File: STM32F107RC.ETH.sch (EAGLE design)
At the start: 30 parts, among them J1 HR911105A, Q1 8MHz, U1 LAN8720A-CP, U2 STM32F107RCT6, X1 CB3LV-3I-74M2500

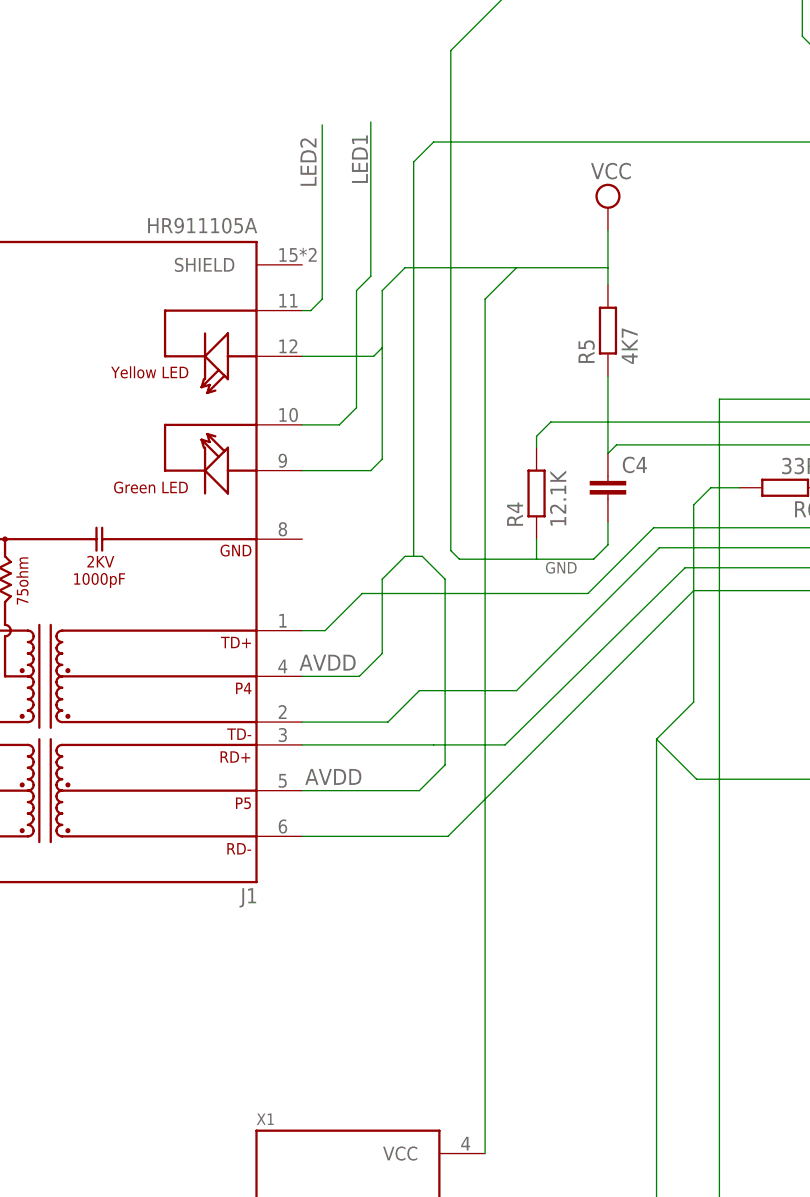
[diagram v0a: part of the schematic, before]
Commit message: Add files via upload
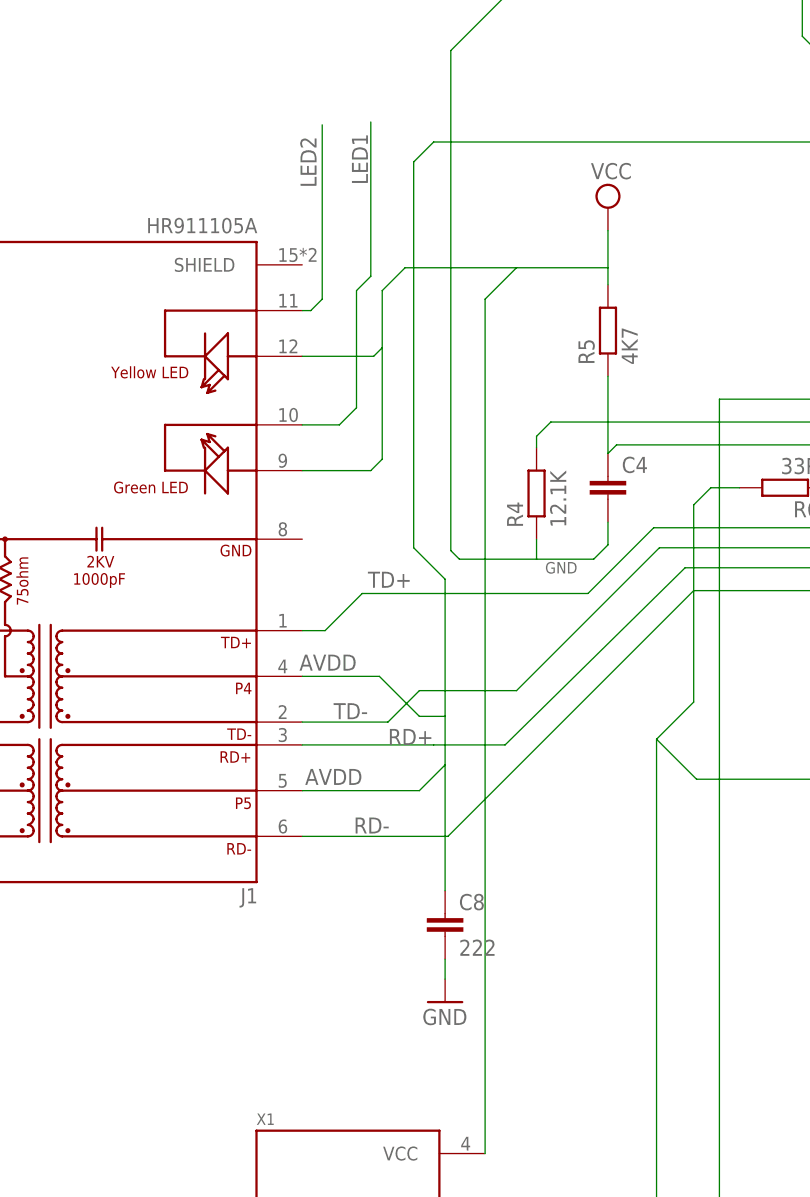
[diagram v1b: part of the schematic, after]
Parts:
- added C8: 222, resistor:C-EUC1206
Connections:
- net N$23 renamed TD+
- net N$28 renamed TD-
- net N$29 renamed RD+
- net N$31 renamed RD-
- net AVDD: now also C8.1
- net GND: now also C8.2
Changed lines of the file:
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@@
 <part name="R13" library="resistor" deviceset="R-EU_" device="0204_7" value="330R"/>
 <part name="R14" library="resistor" deviceset="R-EU_" device="0204_7" value="330R"/>
+<part name="C8" library="resistor" deviceset="C-EU" device="C1206" value="222"/>
+<part name="GND1" library="supply1" deviceset="GND" device=""/>
 </parts>
 <sheets>
@@
 <instance part="R13" gate="G$1" x="-12.3825" y="124.46"/>
 <instance part="R14" gate="G$1" x="-12.3825" y="117.475"/>
+<instance part="C8" gate="G$1" x="-104.14" y="100.33"/>
+<instance part="GND1" gate="1" x="-104.14" y="90.4875"/>
 </instances>
 <busses>
@@
 <junction x="0" y="195.58"/>
 <label x="-9.8425" y="196.5325" size="1.778" layer="95"/>
-<wire x1="-113.665" y1="126.6825" x2="-111.125" y2="129.2225" width="0.1524" layer="91"/>
 <pinref part="J1" gate="G$1" pin="P4"/>
-<wire x1="-120.015" y1="126.6825" x2="-113.665" y2="126.6825" width="0.1524" layer="91"/>
-<wire x1="-111.125" y1="129.2225" x2="-111.125" y2="137.4775" width="0.1524" layer="91"/>
-<wire x1="-111.125" y1="137.4775" x2="-108.585" y2="140.0175" width="0.1524" layer="91"/>
-<wire x1="-104.14" y1="137.4775" x2="-106.68" y2="140.0175" width="0.1524" layer="91"/>
-<wire x1="-104.14" y1="116.84" x2="-104.14" y2="137.4775" width="0.1524" layer="91"/>
+<wire x1="-120.015" y1="126.6825" x2="-111.4425" y2="126.6825" width="0.1524" layer="91"/>
+<wire x1="-104.14" y1="137.4775" x2="-107.6325" y2="140.97" width="0.1524" layer="91"/>
+<wire x1="-104.14" y1="116.84" x2="-104.14" y2="122.2375" width="0.1524" layer="91"/>
 <pinref part="J1" gate="G$1" pin="P5"/>
+<wire x1="-104.14" y1="122.2375" x2="-104.14" y2="137.4775" width="0.1524" layer="91"/>
 <wire x1="-120.015" y1="113.9825" x2="-106.9975" y2="113.9825" width="0.1524" layer="91"/>
 <wire x1="-106.9975" y1="113.9825" x2="-104.14" y2="116.84" width="0.1524" layer="91"/>
-<wire x1="-108.585" y1="140.0175" x2="-107.6325" y2="140.0175" width="0.1524" layer="91"/>
-<wire x1="-107.6325" y1="140.0175" x2="-106.68" y2="140.0175" width="0.1524" layer="91"/>
-<wire x1="-107.6325" y1="140.0175" x2="-107.6325" y2="183.8325" width="0.1524" layer="91"/>
+<wire x1="-107.6325" y1="140.97" x2="-107.6325" y2="183.8325" width="0.1524" layer="91"/>
 <wire x1="-107.6325" y1="183.8325" x2="-105.41" y2="186.055" width="0.1524" layer="91"/>
 <wire x1="-105.41" y1="186.055" x2="-33.02" y2="186.055" width="0.1524" layer="91"/>
@@
 <label x="-120.3325" y="127.3175" size="1.778" layer="95"/>
 <label x="-119.6975" y="114.6175" size="1.778" layer="95"/>
+<wire x1="-111.4425" y1="126.6825" x2="-106.9975" y2="122.2375" width="0.1524" layer="91"/>
+<wire x1="-106.9975" y1="122.2375" x2="-104.14" y2="122.2375" width="0.1524" layer="91"/>
+<wire x1="-104.14" y1="116.84" x2="-104.14" y2="102.87" width="0.1524" layer="91"/>
+<pinref part="C8" gate="G$1" pin="1"/>
 </segment>
 </net>
@@
 <wire x1="29.845" y1="151.4475" x2="35.2425" y2="151.4475" width="0.1524" layer="91"/>
 <label x="30.48" y="149.86" size="1.27" layer="95"/>
+</segment>
+<segment>
+<pinref part="C8" gate="G$1" pin="2"/>
+<pinref part="GND1" gate="1" pin="GND"/>
+<wire x1="-104.14" y1="95.25" x2="-104.14" y2="93.0275" width="0.1524" layer="91"/>
 </segment>
 </net>
@@
 </segment>
 </net>
-<net name="N$23" class="0">
+<net name="TD+" class="0">
 <segment>
 <pinref part="U1" gate="G$1" pin="TXP"/>
@@
 <pinref part="J1" gate="G$1" pin="TD+"/>
 <wire x1="-117.475" y1="131.7625" x2="-120.015" y2="131.7625" width="0.1524" layer="91"/>
-</segment>
-</net>
-<net name="N$28" class="0">
+<label x="-112.7125" y="136.525" size="1.778" layer="95"/>
+</segment>
+</net>
+<net name="TD-" class="0">
 <segment>
 <pinref part="U1" gate="G$1" pin="TXN"/>
@@
 <wire x1="-106.9975" y1="125.095" x2="-110.49" y2="121.6025" width="0.1524" layer="91"/>
 <wire x1="-110.49" y1="121.6025" x2="-120.015" y2="121.6025" width="0.1524" layer="91"/>
-</segment>
-</net>
-<net name="N$29" class="0">
+<label x="-116.5225" y="121.92" size="1.778" layer="95"/>
+</segment>
+</net>
+<net name="RD+" class="0">
 <segment>
 <pinref part="U1" gate="G$1" pin="RXP"/>
@@
 <pinref part="J1" gate="G$1" pin="RD+"/>
 <wire x1="-105.41" y1="119.0625" x2="-120.015" y2="119.0625" width="0.1524" layer="91"/>
-</segment>
-</net>
-<net name="N$31" class="0">
+<label x="-110.49" y="119.0625" size="1.778" layer="95"/>
+</segment>
+</net>
+<net name="RD-" class="0">
 <segment>
 <pinref part="U1" gate="G$1" pin="RXN"/>
@@
 <pinref part="J1" gate="G$1" pin="RD-"/>
 <wire x1="-103.8225" y1="108.9025" x2="-120.015" y2="108.9025" width="0.1524" layer="91"/>
-</segment>
-</net>
+<label x="-114.3" y="109.22" size="1.778" layer="95"/>
+</segment>
+</net>

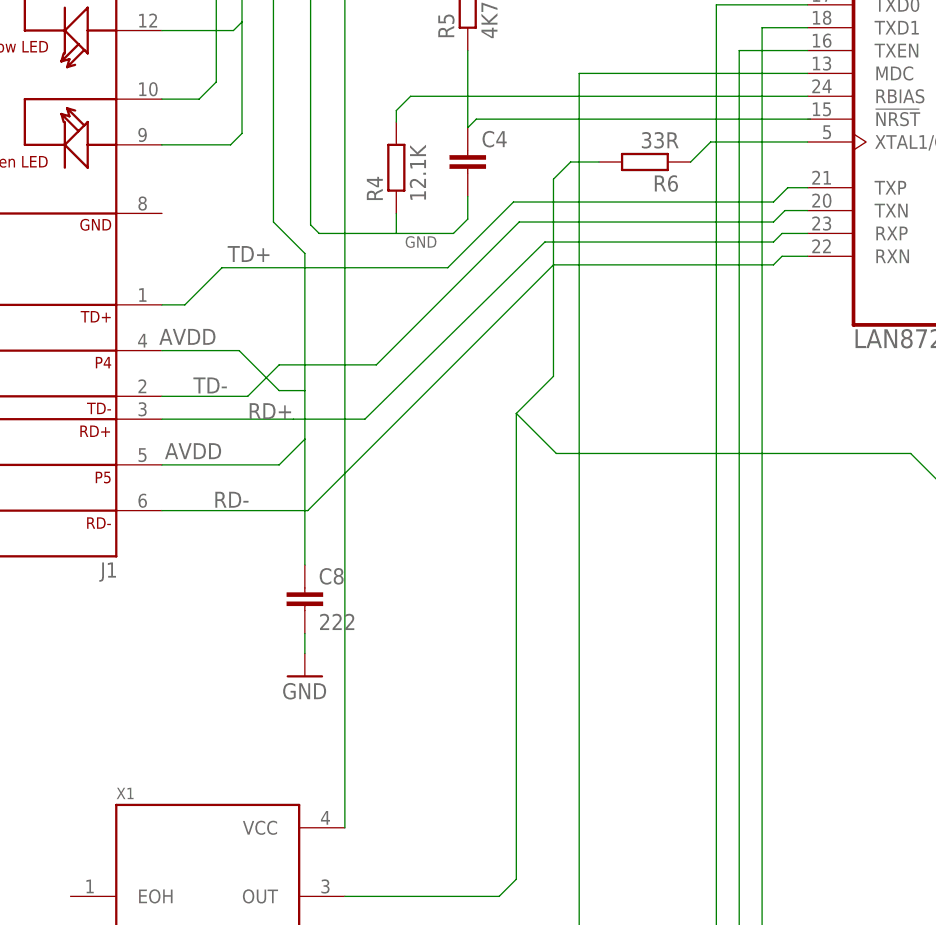
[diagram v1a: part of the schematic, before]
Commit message: Add files via upload
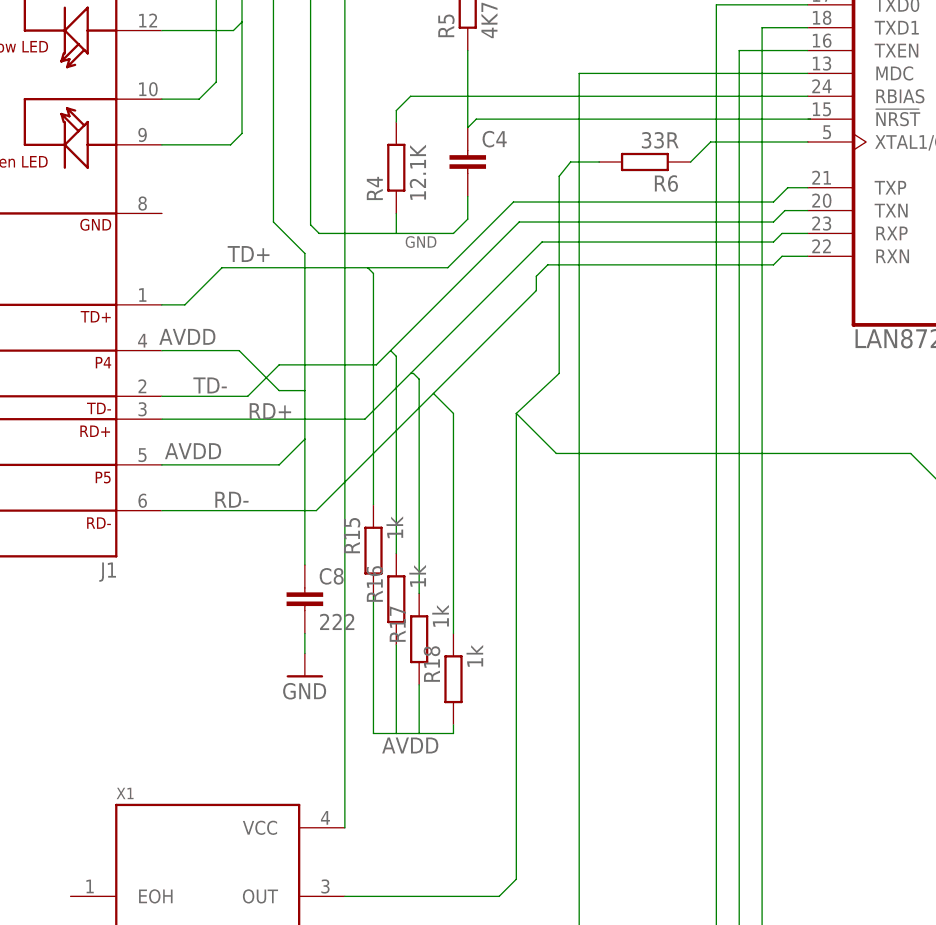
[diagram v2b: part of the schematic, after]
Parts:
- added R15, R16, R17, R18: 1k, resistor:R-EU_0204_7
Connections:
- net AVDD: now also R15.2, R16.2, R17.2, R18.2
- net RD+: now also R17.1
- net RD-: now also R18.1
- net TD+: now also R15.1
- net TD-: now also R16.1
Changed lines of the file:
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@@
 <part name="C8" library="resistor" deviceset="C-EU" device="C1206" value="222"/>
 <part name="GND1" library="supply1" deviceset="GND" device=""/>
+<part name="R15" library="resistor" deviceset="R-EU_" device="0204_7" value="1k"/>
+<part name="R16" library="resistor" deviceset="R-EU_" device="0204_7" value="1k"/>
+<part name="R17" library="resistor" deviceset="R-EU_" device="0204_7" value="1k"/>
+<part name="R18" library="resistor" deviceset="R-EU_" device="0204_7" value="1k"/>
 </parts>
 <sheets>
@@
 <instance part="C8" gate="G$1" x="-104.14" y="100.33"/>
 <instance part="GND1" gate="1" x="-104.14" y="90.4875"/>
+<instance part="R15" gate="G$1" x="-96.52" y="104.4575" rot="MR270"/>
+<instance part="R16" gate="G$1" x="-93.98" y="99.06" rot="MR270"/>
+<instance part="R17" gate="G$1" x="-91.44" y="94.615" rot="MR270"/>
+<instance part="R18" gate="G$1" x="-87.63" y="90.17" rot="MR270"/>
 </instances>
 <busses>
@@
 <pinref part="C8" gate="G$1" pin="1"/>
 </segment>
+<segment>
+<pinref part="R17" gate="G$1" pin="2"/>
+<wire x1="-91.44" y1="89.535" x2="-91.44" y2="84.1375" width="0.1524" layer="91"/>
+<wire x1="-91.44" y1="84.1375" x2="-87.63" y2="84.1375" width="0.1524" layer="91"/>
+<pinref part="R18" gate="G$1" pin="2"/>
+<wire x1="-87.63" y1="84.1375" x2="-87.63" y2="85.09" width="0.1524" layer="91"/>
+<pinref part="R16" gate="G$1" pin="2"/>
+<wire x1="-93.98" y1="93.98" x2="-93.98" y2="84.1375" width="0.1524" layer="91"/>
+<wire x1="-93.98" y1="84.1375" x2="-91.44" y2="84.1375" width="0.1524" layer="91"/>
+<pinref part="R15" gate="G$1" pin="2"/>
+<wire x1="-96.52" y1="99.3775" x2="-96.52" y2="84.1375" width="0.1524" layer="91"/>
+<wire x1="-96.52" y1="84.1375" x2="-93.98" y2="84.1375" width="0.1524" layer="91"/>
+<label x="-95.5675" y="81.915" size="1.778" layer="95"/>
+</segment>
 </net>
 <net name="N$12" class="0">
@@
 <pinref part="R6" gate="G$1" pin="2"/>
 <wire x1="-71.4375" y1="147.6375" x2="-74.6125" y2="147.6375" width="0.1524" layer="91"/>
-<wire x1="-74.6125" y1="147.6375" x2="-76.5175" y2="145.7325" width="0.1524" layer="91"/>
-<wire x1="-76.5175" y1="145.7325" x2="-76.5175" y2="123.825" width="0.1524" layer="91"/>
-<wire x1="-76.5175" y1="123.825" x2="-80.645" y2="119.6975" width="0.1524" layer="91"/>
+<wire x1="-74.6125" y1="147.6375" x2="-75.8825" y2="146.05" width="0.1524" layer="91"/>
+<wire x1="-75.8825" y1="146.05" x2="-75.8825" y2="124.1425" width="0.1524" layer="91"/>
+<wire x1="-75.8825" y1="124.1425" x2="-80.645" y2="119.6975" width="0.1524" layer="91"/>
 <wire x1="-80.645" y1="119.6975" x2="-76.2" y2="115.2525" width="0.1524" layer="91"/>
 <wire x1="-76.2" y1="115.2525" x2="-36.83" y2="115.2525" width="0.1524" layer="91"/>
@@
 <wire x1="-52.07" y1="143.1925" x2="-80.9625" y2="143.1925" width="0.1524" layer="91"/>
 <wire x1="-80.9625" y1="143.1925" x2="-88.265" y2="135.89" width="0.1524" layer="91"/>
-<wire x1="-88.265" y1="135.89" x2="-113.3475" y2="135.89" width="0.1524" layer="91"/>
+<wire x1="-88.265" y1="135.89" x2="-97.155" y2="135.89" width="0.1524" layer="91"/>
+<wire x1="-97.155" y1="135.89" x2="-113.3475" y2="135.89" width="0.1524" layer="91"/>
 <wire x1="-113.3475" y1="135.89" x2="-117.475" y2="131.7625" width="0.1524" layer="91"/>
 <pinref part="J1" gate="G$1" pin="TD+"/>
 <wire x1="-117.475" y1="131.7625" x2="-120.015" y2="131.7625" width="0.1524" layer="91"/>
 <label x="-112.7125" y="136.525" size="1.778" layer="95"/>
+<pinref part="R15" gate="G$1" pin="1"/>
+<wire x1="-96.52" y1="109.5375" x2="-96.52" y2="135.255" width="0.1524" layer="91"/>
+<wire x1="-96.52" y1="135.255" x2="-97.155" y2="135.89" width="0.1524" layer="91"/>
 </segment>
 </net>
@@
 <wire x1="-50.8" y1="142.24" x2="-52.07" y2="140.97" width="0.1524" layer="91"/>
 <wire x1="-52.07" y1="140.97" x2="-80.3275" y2="140.97" width="0.1524" layer="91"/>
-<wire x1="-80.3275" y1="140.97" x2="-96.2025" y2="125.095" width="0.1524" layer="91"/>
+<wire x1="-80.3275" y1="140.97" x2="-94.615" y2="126.6825" width="0.1524" layer="91"/>
+<wire x1="-94.615" y1="126.6825" x2="-96.2025" y2="125.095" width="0.1524" layer="91"/>
 <wire x1="-96.2025" y1="125.095" x2="-106.9975" y2="125.095" width="0.1524" layer="91"/>
 <pinref part="J1" gate="G$1" pin="TD-"/>
@@
 <wire x1="-110.49" y1="121.6025" x2="-120.015" y2="121.6025" width="0.1524" layer="91"/>
 <label x="-116.5225" y="121.92" size="1.778" layer="95"/>
+<pinref part="R16" gate="G$1" pin="1"/>
+<wire x1="-93.98" y1="104.14" x2="-93.98" y2="126.0475" width="0.1524" layer="91"/>
+<wire x1="-93.98" y1="126.0475" x2="-94.615" y2="126.6825" width="0.1524" layer="91"/>
 </segment>
 </net>
@@
 <wire x1="-48.26" y1="139.7" x2="-51.1175" y2="139.7" width="0.1524" layer="91"/>
 <wire x1="-51.1175" y1="139.7" x2="-52.07" y2="138.7475" width="0.1524" layer="91"/>
-<wire x1="-52.07" y1="138.7475" x2="-77.47" y2="138.7475" width="0.1524" layer="91"/>
-<wire x1="-77.47" y1="138.7475" x2="-97.4725" y2="119.0625" width="0.1524" layer="91"/>
-<wire x1="-97.4725" y1="119.0625" x2="-105.41" y2="119.0625" width="0.1524" layer="91"/>
+<wire x1="-52.07" y1="138.7475" x2="-77.7875" y2="138.7475" width="0.1524" layer="91"/>
 <pinref part="J1" gate="G$1" pin="RD+"/>
-<wire x1="-105.41" y1="119.0625" x2="-120.015" y2="119.0625" width="0.1524" layer="91"/>
+<wire x1="-97.4725" y1="119.0625" x2="-120.015" y2="119.0625" width="0.1524" layer="91"/>
 <label x="-110.49" y="119.0625" size="1.778" layer="95"/>
+<wire x1="-97.4725" y1="119.0625" x2="-92.3925" y2="124.1425" width="0.1524" layer="91"/>
+<wire x1="-92.3925" y1="124.1425" x2="-77.7875" y2="138.7475" width="0.1524" layer="91"/>
+<wire x1="-91.44" y1="123.5075" x2="-92.075" y2="124.1425" width="0.1524" layer="91"/>
+<pinref part="R17" gate="G$1" pin="1"/>
+<wire x1="-91.44" y1="99.695" x2="-91.44" y2="123.5075" width="0.1524" layer="91"/>
+<wire x1="-92.075" y1="124.1425" x2="-92.3925" y2="124.1425" width="0.1524" layer="91"/>
 </segment>
 </net>
@@
 <wire x1="-48.26" y1="137.16" x2="-51.1175" y2="137.16" width="0.1524" layer="91"/>
 <wire x1="-51.1175" y1="137.16" x2="-52.07" y2="136.2075" width="0.1524" layer="91"/>
-<wire x1="-52.07" y1="136.2075" x2="-76.5175" y2="136.2075" width="0.1524" layer="91"/>
-<wire x1="-76.5175" y1="136.2075" x2="-103.8225" y2="108.9025" width="0.1524" layer="91"/>
+<wire x1="-52.07" y1="136.2075" x2="-77.1525" y2="136.2075" width="0.1524" layer="91"/>
 <pinref part="J1" gate="G$1" pin="RD-"/>
-<wire x1="-103.8225" y1="108.9025" x2="-120.015" y2="108.9025" width="0.1524" layer="91"/>
+<wire x1="-102.87" y1="108.9025" x2="-120.015" y2="108.9025" width="0.1524" layer="91"/>
 <label x="-114.3" y="109.22" size="1.778" layer="95"/>
-</segment>
-</net>
+<wire x1="-102.87" y1="108.9025" x2="-89.8525" y2="121.92" width="0.1524" layer="91"/>
+<wire x1="-89.8525" y1="121.92" x2="-78.4225" y2="133.35" width="0.1524" layer="91"/>
+<wire x1="-78.4225" y1="133.35" x2="-78.4225" y2="134.9375" width="0.1524" layer="91"/>
+<wire x1="-78.4225" y1="134.9375" x2="-77.1525" y2="136.2075" width="0.1524" layer="91"/>
+<pinref part="R18" gate="G$1" pin="1"/>
+<wire x1="-87.63" y1="95.25" x2="-87.63" y2="119.6975" width="0.1524" layer="91"/>
+<wire x1="-87.63" y1="119.6975" x2="-89.8525" y2="121.92" width="0.1524" layer="91"/>
+</segment>
+</net>
